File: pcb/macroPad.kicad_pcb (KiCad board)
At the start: 2 copper layers, 83 x 41 mm, 8 parts, among them SW1 SW_Push, SW2 SW_Push, SW3 SW_Push, SW4 SW_Push, SW5 SW_Push, SW6 RotaryEncoder_Switch, U1 MOUDLE-SEEEDUINO-XIAO, U2 ER_OLEDM0.91_1x-I2C

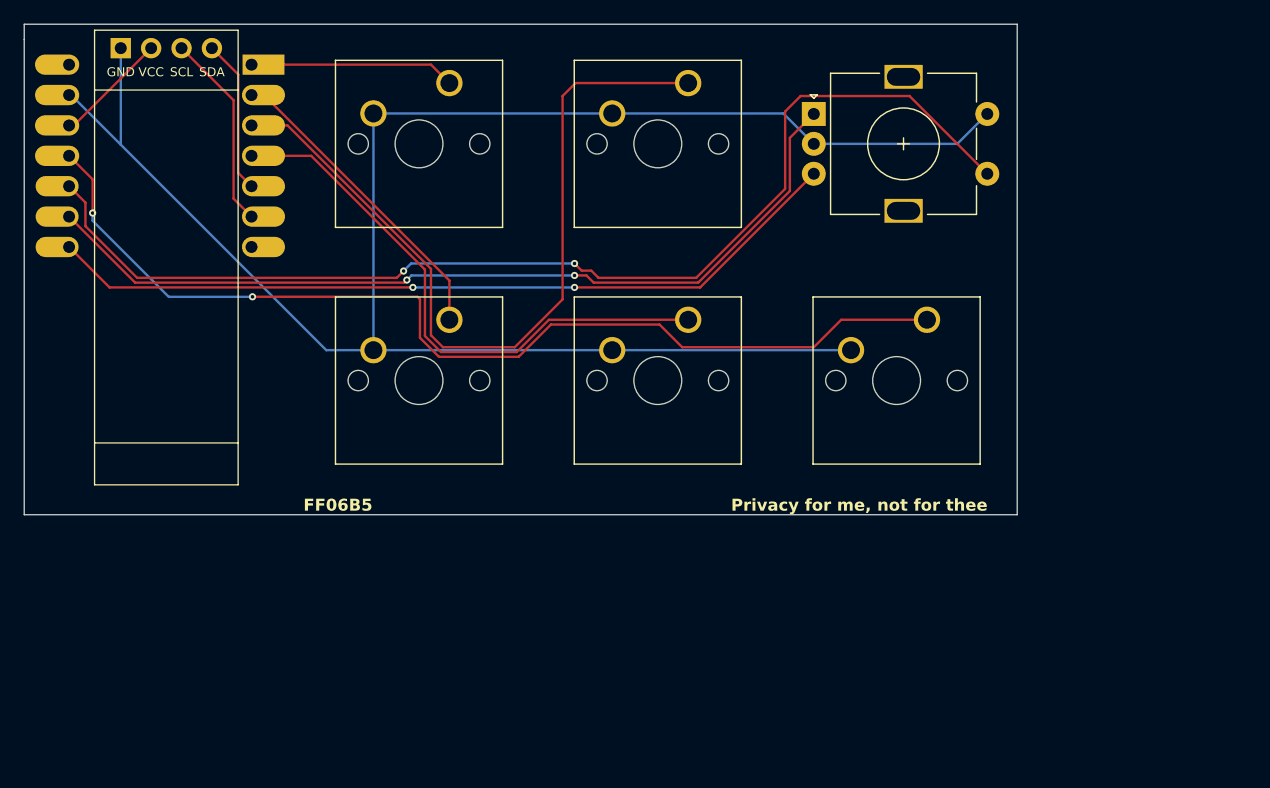
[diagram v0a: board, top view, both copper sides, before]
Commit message: Replace w/ Updated Design
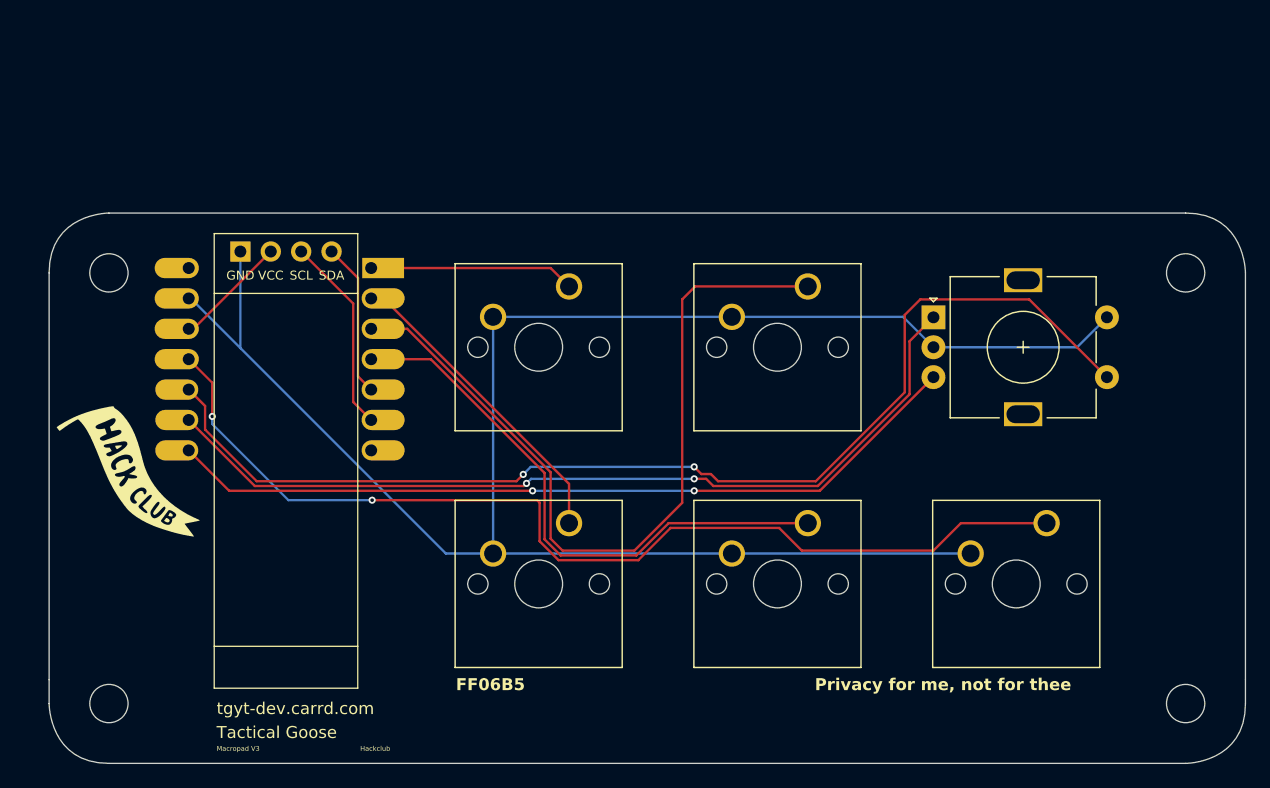
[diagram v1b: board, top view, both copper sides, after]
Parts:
- added G***: LOGO, LOGO, F.Cu at (90.0, 101.0)
- added H1: MountingHole, MountingHole:MountingHole_3.2mm_M3, F.Cu at (178.0, 84.0)
- added H2: MountingHole, MountingHole:MountingHole_3.2mm_M3, F.Cu at (178.0, 120.0)
- added H3: MountingHole, MountingHole:MountingHole_3.2mm_M3, F.Cu at (88.0, 84.0)
- added H4: MountingHole, MountingHole:MountingHole_3.2mm_M3, F.Cu at (88.0, 120.0)
- moved SW1 19.7 mm to (126.5, 85.1)
- moved SW2 19.7 mm to (126.5, 104.9)
- moved SW3 19.7 mm to (146.4, 85.1)
- moved SW4 19.7 mm to (146.4, 104.9)
- moved SW5 19.7 mm to (166.4, 104.9)
- moved SW6 19.7 mm to (156.9, 87.7)
- moved U1 19.7 mm to (102.3, 91.2)
- moved U2 19.7 mm to (96.8, 118.7)
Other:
- board size 83 x 41 mm -> 100 x 46 mm
